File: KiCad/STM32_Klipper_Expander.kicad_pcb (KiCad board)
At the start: 2 copper layers, 100 x 24 mm, 47 parts, among them J1 USB_B_Micro, J10 Conn_01x01, J11 Conn_01x03, J12 Conn_01x02, J2 Conn_01x04, J4 Conn_01x03, J5 Vin, J6 Screw_Terminal_01x08, J7 Conn_01x02, J8 Conn_01x02, J9 Conn_01x02, Q1 IRLML6344TRPBF, Q2 IRLML6344TRPBF, Q3 IRLML6344TRPBF, Q4 IRLML6344TRPBF, SW2 SW_SPST, U1 STM32F042F6Px, U2 AP2127K-3.3, U3 74LVC1G17

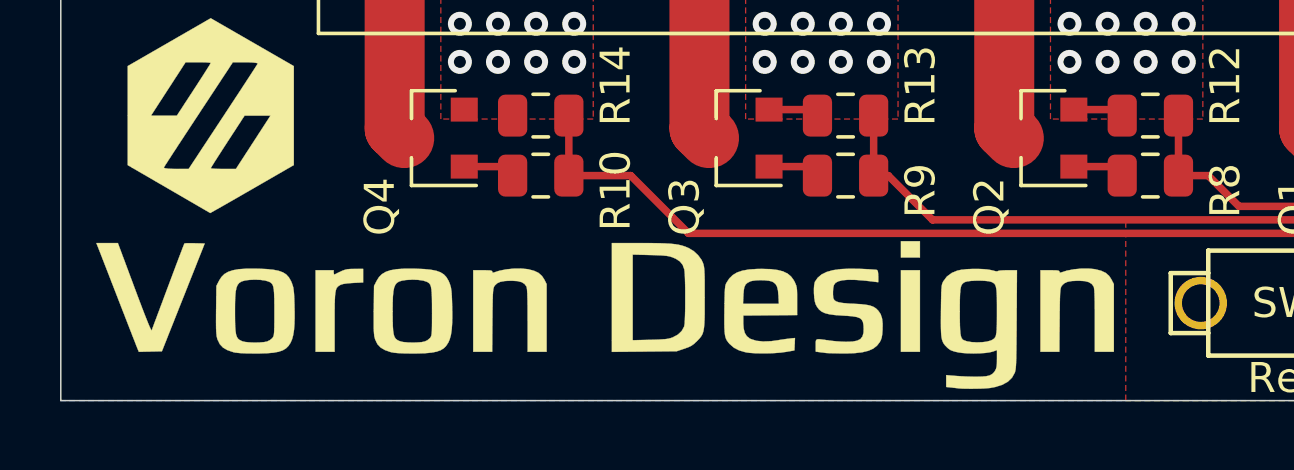
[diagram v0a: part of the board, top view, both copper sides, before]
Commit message: file organization
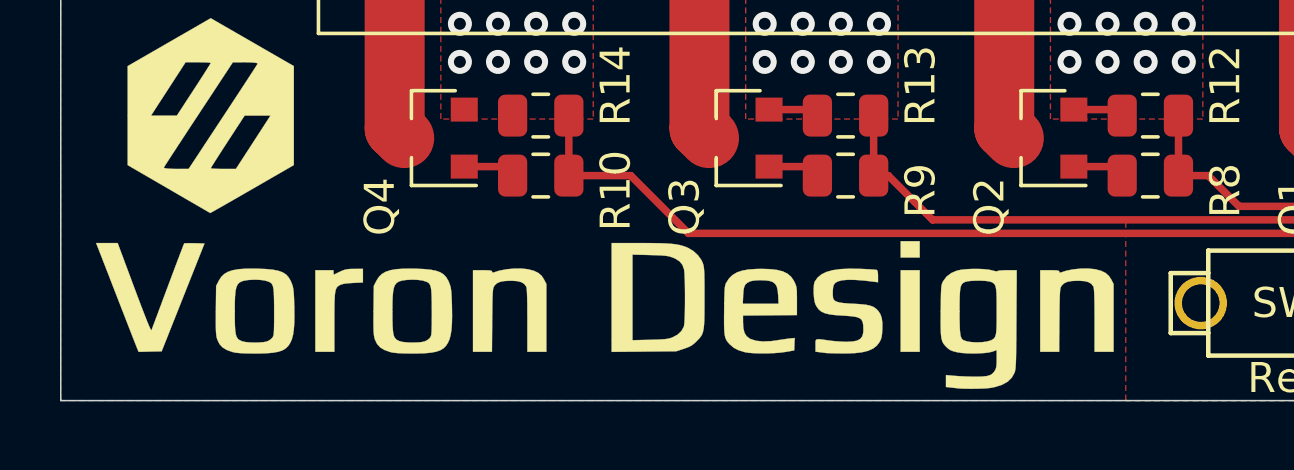
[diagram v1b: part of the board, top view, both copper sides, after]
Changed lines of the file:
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@@
   )
   (module TRA_KiCad_Footprints:VoronDesign_Text_35x20 locked (layer F.Cu)
-    (at 118.25 96.5)
+    (at 118.242 96.5)
     (fp_text reference G*** (at 0 0) (layer F.SilkS) hide
       (effects (font (size 1.524 1.524) (thickness 0.3)))
